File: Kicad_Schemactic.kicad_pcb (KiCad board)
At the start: 2 copper layers, 100 x 150 mm, 15 parts, among them J1 BME 280, J10 BOOST, J11 Hall effect, J12 DHT11, J13 RTC, J2 MQ 135, J3 PMY 2.5, J4 water sensor, J5 IR sensor, J6 Sound Sensor, J7 IR sensor, J8 Tp4056, J9 Battery, U1 ESP32-S3-DEVKITC-1U-N8R2, U3 Oled display

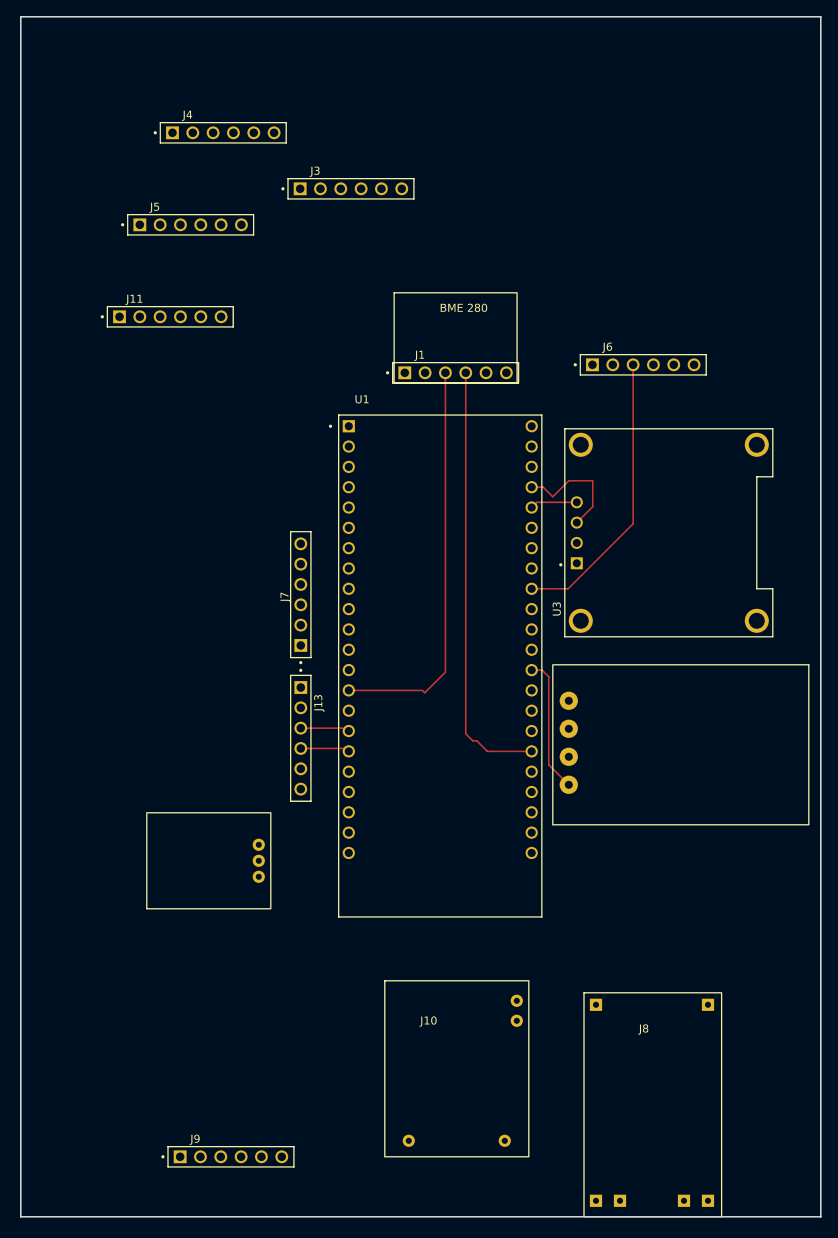
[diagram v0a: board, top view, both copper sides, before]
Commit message: Add files via upload
sd
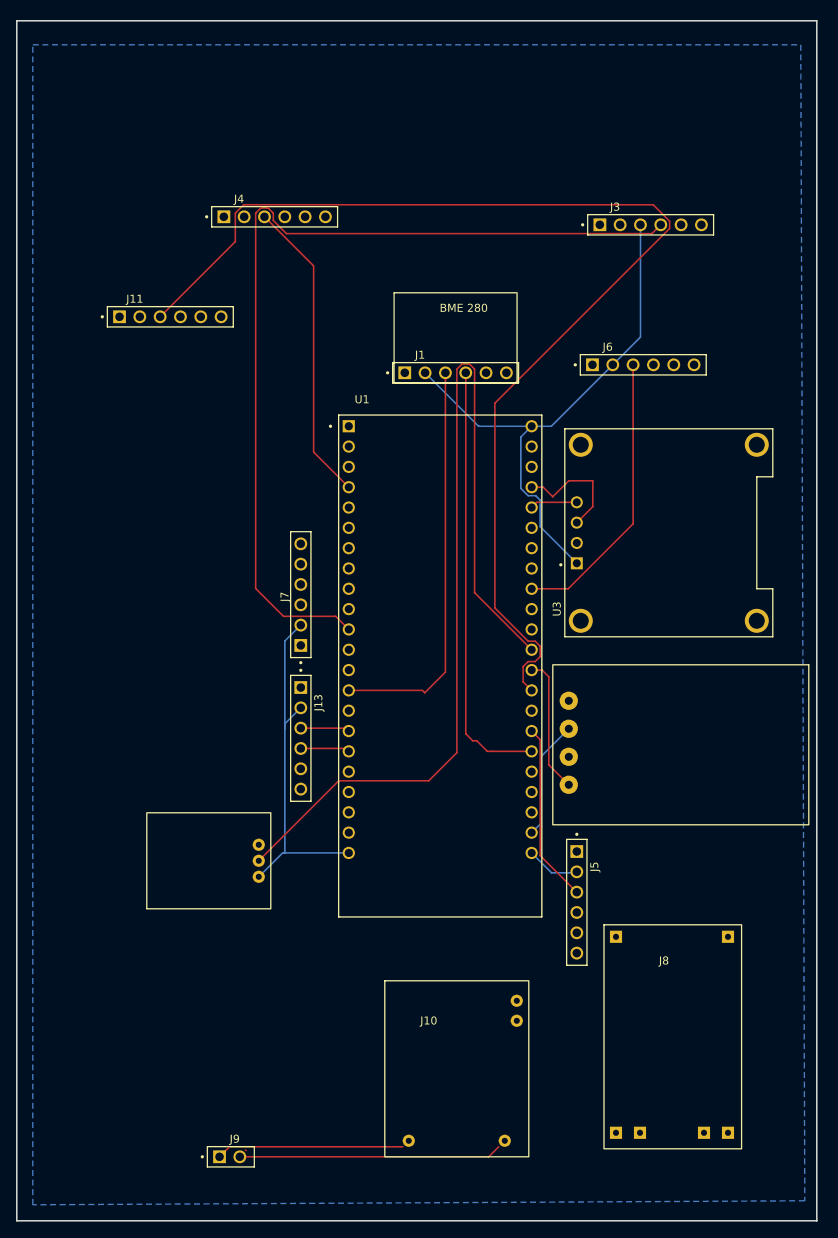
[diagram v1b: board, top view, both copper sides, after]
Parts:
- moved J5 97.5 mm to (122.5, 154.2), turned to -90 degrees
- moved J3 37.7 mm to (131.7, 69.5)
- moved J4 12.3 mm to (84.7, 68.5)
- moved J8 8.86 mm to (133.4, 163.0)
- moved J9 4.92 mm to (84.2, 186.0)
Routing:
- net Net-(J11-OUT): track 0.00 -> 144.8 mm
- net GND: track 0.00 -> 136.4 mm
- net Net-(J12-DATA): track 0.00 -> 119.1 mm
- net Net-(U1-GPIO18): track 0.00 -> 113.9 mm
- net Net-(J4-D0): track 0.00 -> 38.2 mm
- net Net-(J10--BAT): track 0.00 -> 32.9 mm
- net Net-(J10-+BAT): track 0.00 -> 23.4 mm
- net Net-(J5-OUT): track 0.00 -> 22.5 mm
- added copper zone on B.Cu, net GND
